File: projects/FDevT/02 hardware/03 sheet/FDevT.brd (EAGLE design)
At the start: 100 x 80 mm, 19 parts, among them IC2 LP2950

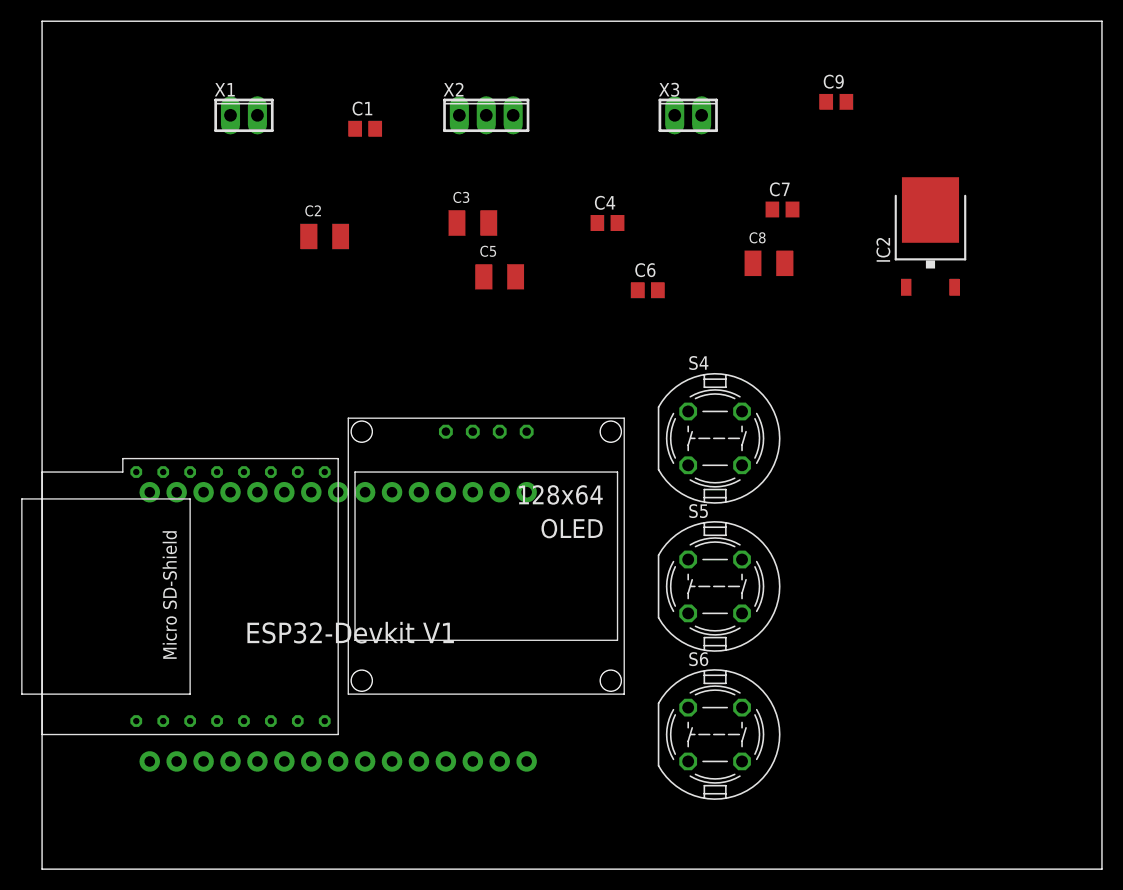
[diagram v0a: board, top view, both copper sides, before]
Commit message: final Version
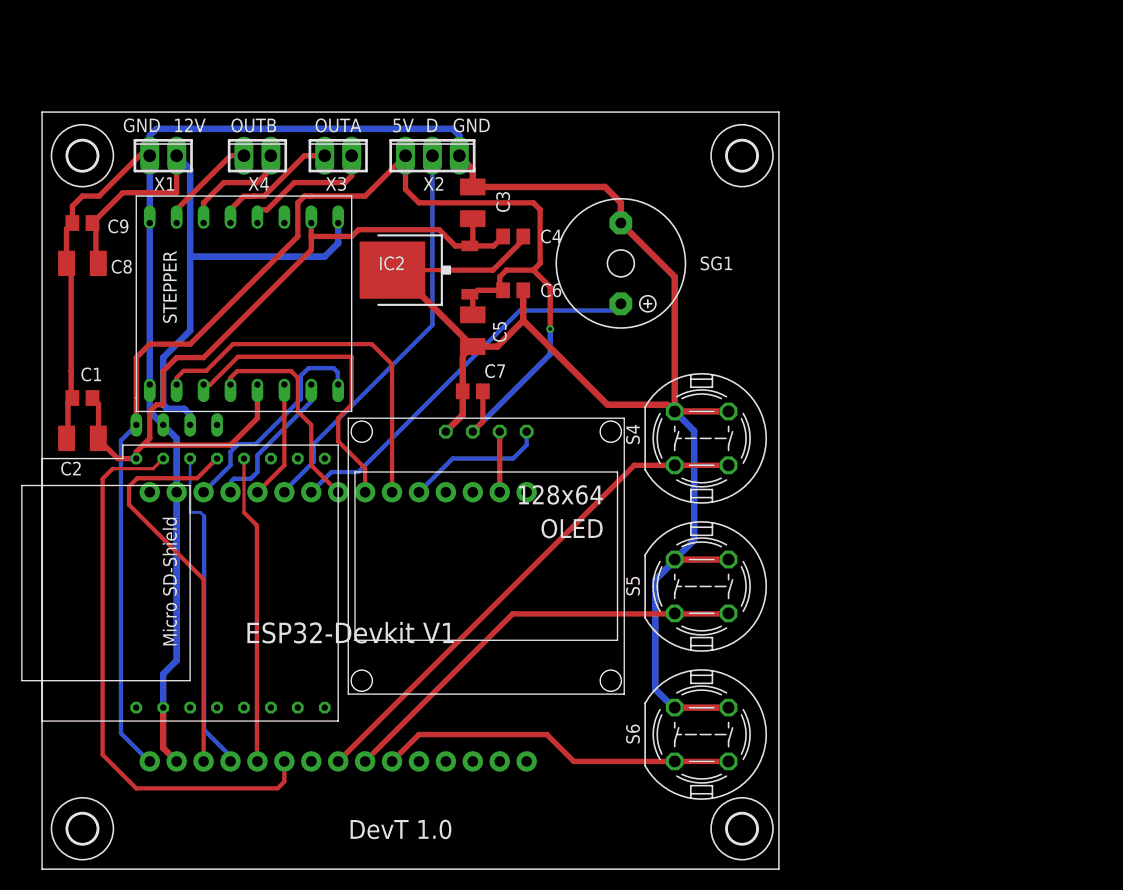
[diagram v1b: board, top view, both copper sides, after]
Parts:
- added SG1: F/TMB, buzzer:F/TMB
- added STEPPER: TBB6612, TBB6612d:DRIVER
- added U$4: STEPUP, AMESYS_neu:STEPUP
- added U$5, U$6, U$7, U$8: (no value), holes:2,8
- added X4: OUTB, con-phoenix-254:2POL254
- C1, C4, C6, C7, C9: value (none) -> 100n
- C2, C3, C5, C8: value (none) -> 10µ
- X1: value (none) -> IN
- X2: value (none) -> Motor
- X3: value (none) -> OUTA
- moved C9 72.0 mm to (3.81, 61.0), turned to 180 degrees
- moved C8 64.8 mm to (3.81, 57.1), turned to 180 degrees
- moved IC2 48.4 mm to (35.6, 56.5), turned to 90 degrees
- moved C1 36.8 mm to (3.81, 44.5), turned to 180 degrees
- moved C7 33.9 mm to (40.6, 45.1), turned to 180 degrees
- moved X3 33.2 mm to (27.9, 67.3)
- moved C2 29.8 mm to (3.81, 40.6), turned to 180 degrees
- moved C6 12.7 mm to (44.5, 54.6)
- moved C4 8.98 mm to (44.5, 59.7)
- moved X1 8.52 mm to (11.4, 67.3)
- moved X2 6.35 mm to (36.8, 67.3)
- moved C5 5.68 mm to (40.6, 50.8), turned to 270 degrees
- moved C3 1.91 mm to (40.6, 62.9), turned to 90 degrees
- moved S4 1.27 mm to (62.2, 40.6)
- moved S5 1.27 mm to (62.2, 26.7)
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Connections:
- removed net R_CHANGE: BOARD1.D2
- new net AIN1: BOARD1.D2, STEPPER.10
- new net AIN2: BOARD1.D4, STEPPER.11
- new net N$3: STEPPER.5, X3.2
- new net N$4: STEPPER.4, X3.1
- new net N$5: BOARD1.D5, STEPPER.13
- new net N$6: BOARD1.D18, STEPPER.14
- new net N$7: BOARD1.D19, STEPPER.15
- new net N$8: STEPPER.3, X4.2
- new net N$9: STEPPER.2, X4.1
- net +12V: now also STEPPER.8, U$4.IN
- net +3V3: now also STEPPER.12, STEPPER.7
- net +5V: now also U$4.OUT
- net BEEP: now also BOARD1.D17, SG1.+; no longer BOARD1.D4
- net GND: now also SG1.-, STEPPER.1, STEPPER.16, U$4.GND
- net PWM: now also STEPPER.9
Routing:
- net GND: track 0.00 -> 275.8 mm
- net +5V: track 0.00 -> 132.8 mm, vias 0 -> 1
- net +3V3: track 0.00 -> 77.0 mm
- net +12V: track 0.00 -> 62.5 mm
- net CS: track 0.00 -> 53.2 mm
- net DOWN: track 0.00 -> 48.5 mm
- net ENTER: track 0.00 -> 40.3 mm
- net MISO: track 0.00 -> 38.3 mm
- net DRIVE: track 0.00 -> 37.5 mm
- net BEEP: track 0.00 -> 36.6 mm
- net N$7: track 0.00 -> 35.1 mm
- net UP: track 0.00 -> 34.1 mm
- net MOSI: track 0.00 -> 30.7 mm
- net N$6: track 0.00 -> 29.4 mm
- net SCK: track 0.00 -> 29.1 mm
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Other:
- board size 100 x 80 mm -> 69.5 x 71.4 mm
- board text added: "12V"
- board text added: "5V"
- board text added: "D"
- board text added: "DevT 1.0"
- board text added: "GND"
- board text added: "OUTA"
- board text added: "OUTB"
